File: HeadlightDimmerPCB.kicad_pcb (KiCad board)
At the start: 2 copper layers, 24 x 18 mm, 12 parts, among them J1 Conn_02x02_Counter_Clockwise, Q1 NMOS, U1 LMC555xTP

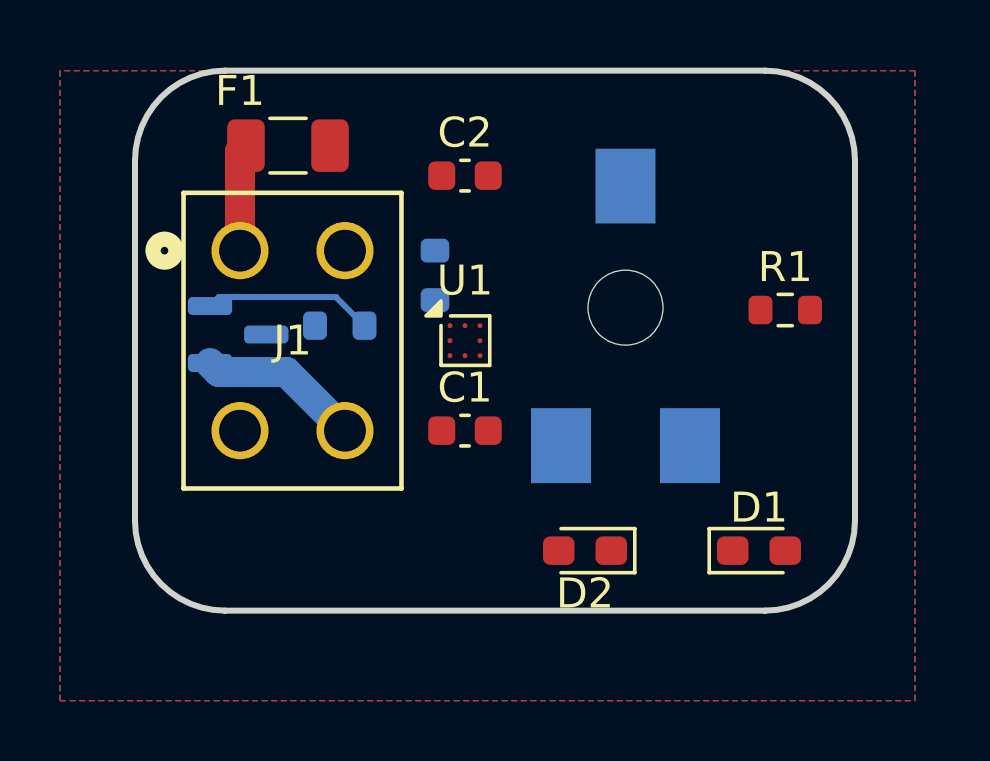
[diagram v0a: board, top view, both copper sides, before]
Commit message: bah
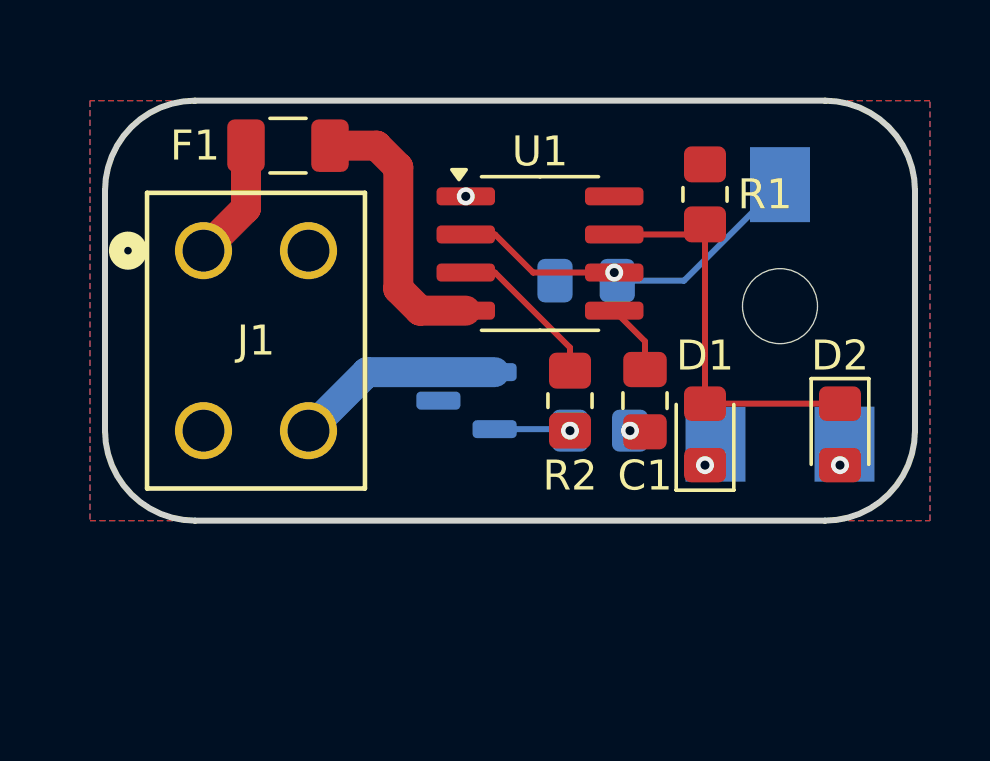
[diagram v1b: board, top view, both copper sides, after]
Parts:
- C1: footprint Capacitor_SMD:C_0603_1608Metric -> Capacitor_SMD:C_0805_2012Metric_Pad1.18x1.45mm_HandSolder
- C2: footprint Capacitor_SMD:C_0603_1608Metric -> Capacitor_SMD:C_0805_2012Metric_Pad1.18x1.45mm_HandSolder; moved to B.Cu
- D1, D2: footprint Diode_SMD:D_0603_1608Metric_Pad1.05x0.95mm_HandSolder -> Diode_SMD:D_0805_2012Metric_Pad1.15x1.40mm_HandSolder
- R1, R3: footprint Resistor_SMD:R_0603_1608Metric -> Resistor_SMD:R_0805_2012Metric_Pad1.20x1.40mm_HandSolder
- R2: footprint Resistor_SMD:R_0603_1608Metric -> Resistor_SMD:R_0805_2012Metric_Pad1.20x1.40mm_HandSolder; moved to F.Cu
- U1: value LMC555xTP -> LMC555xM; footprint Package_BGA:Texas_DSBGA-8_1.43x1.41mm_Layout3x3_P0.5mm -> Package_SO:SOIC-8_3.9x4.9mm_P1.27mm
- moved R3 9.35 mm to (158.5, 94.0), turned to 0 degrees
- moved D2 9.34 mm to (166.5, 94.1), turned to -90 degrees
- moved Q1 7.93 mm to (154.1, 93.0), turned to 180 degrees
- moved R2 6.14 mm to (157.5, 93.0), turned to -90 degrees
- moved C1 6.08 mm to (160.0, 93.0), turned to -90 degrees
- moved C2 5.34 mm to (158.0, 89.0), turned to 180 degrees
- moved RV1 5.15 mm to (164.5, 90.1)
- moved R1 4.69 mm to (162.0, 86.1), turned to 90 degrees
- moved D1 4.27 mm to (162.0, 94.1), turned to 90 degrees
- moved U1 3.83 mm to (156.5, 88.1)
- moved J1 1.22 mm to (145.3, 88.0)
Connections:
- R1 pad 2: VBC -> VDC
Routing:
- net /DIS: track 0.00 -> 13.6 mm
- net Net-(U1-THR): track 0.00 -> 12.2 mm, vias 0 -> 1
- net VDC: track 0.00 -> 9.18 mm
- net Net-(U1-Q): track 0.00 -> 5.28 mm
- net Net-(Q1-G): track 5.67 -> 2.53 mm, vias 0 -> 1
- net Net-(U1-CV): track 0.00 -> 2.39 mm
- net /HL_OUT: track 5.43 -> 7.01 mm
- net Net-(D1-K): track 0.00 -> 0.84 mm, vias 0 -> 1
- net Net-(D2-A): track 0.00 -> 0.76 mm, vias 0 -> 1
- net +12V: track 3.58 -> 4.09 mm
- net GNDPWR: vias 0 -> 2
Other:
- board size 24 x 18 mm -> 27 x 14 mm
- board text added: "UTSVT Headlight Dimmer PCB Summer 2025 Parthiv Shah"
